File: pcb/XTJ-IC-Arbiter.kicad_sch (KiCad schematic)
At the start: 34 parts, among them J3 DTM13-12PA-R008, SW1 SW_DIP_x01, SW2 SW_DIP_x01, U1 LM2672N-5.0, U3 Teensy4.0, U4 MCP2562-H-P, U5 SP723ABG

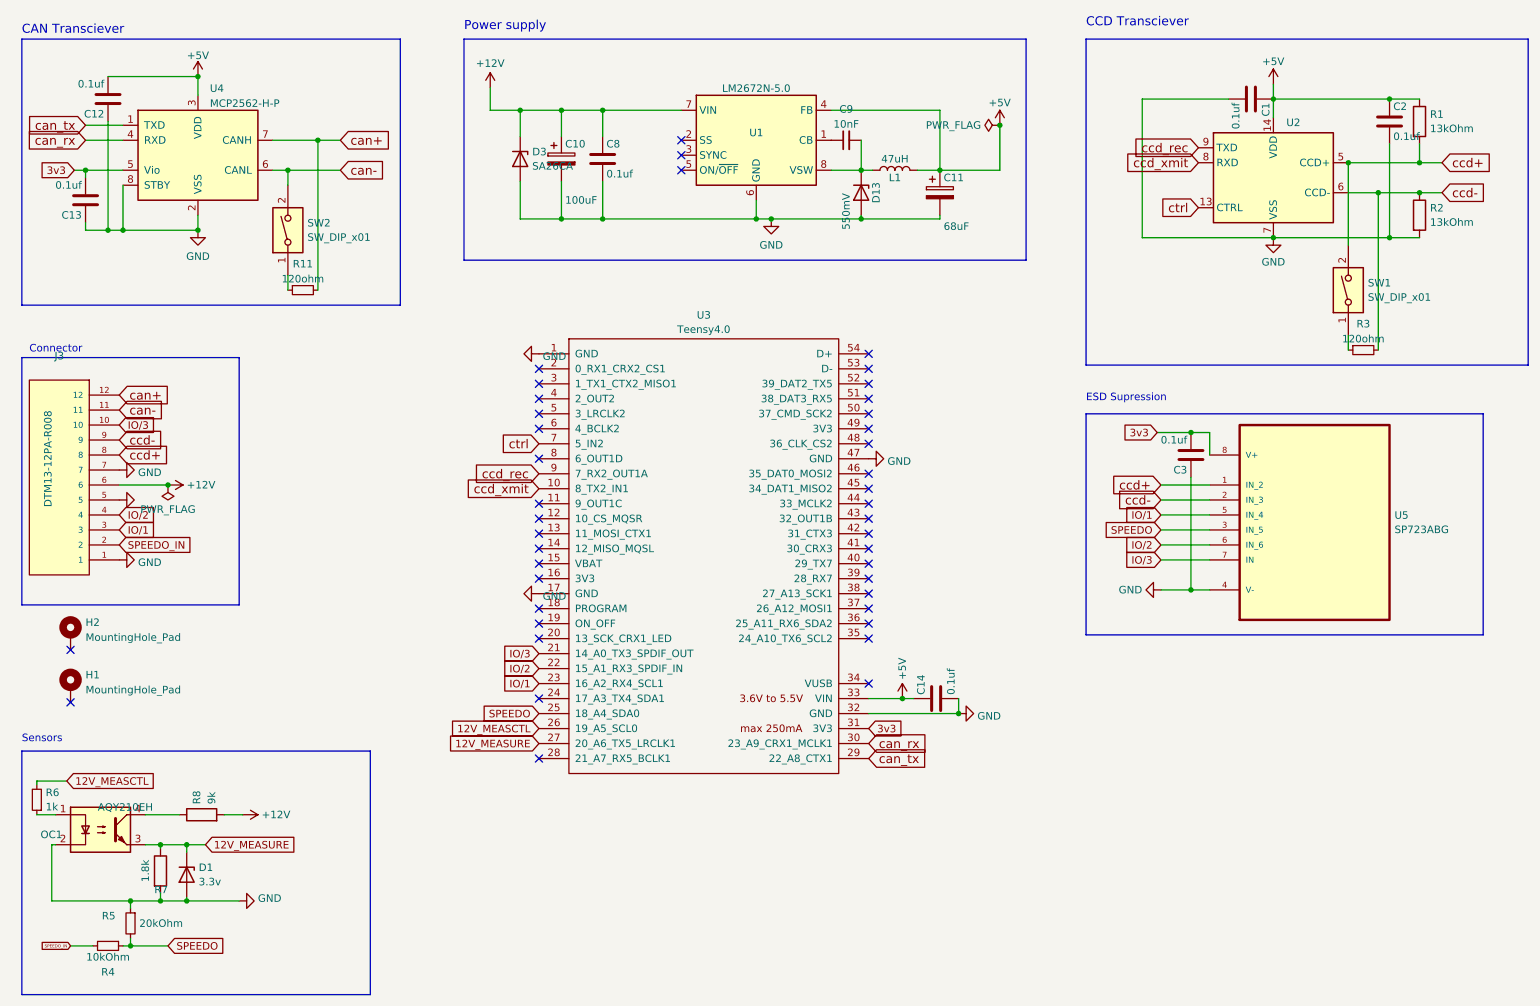
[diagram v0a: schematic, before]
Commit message: ugly but functional
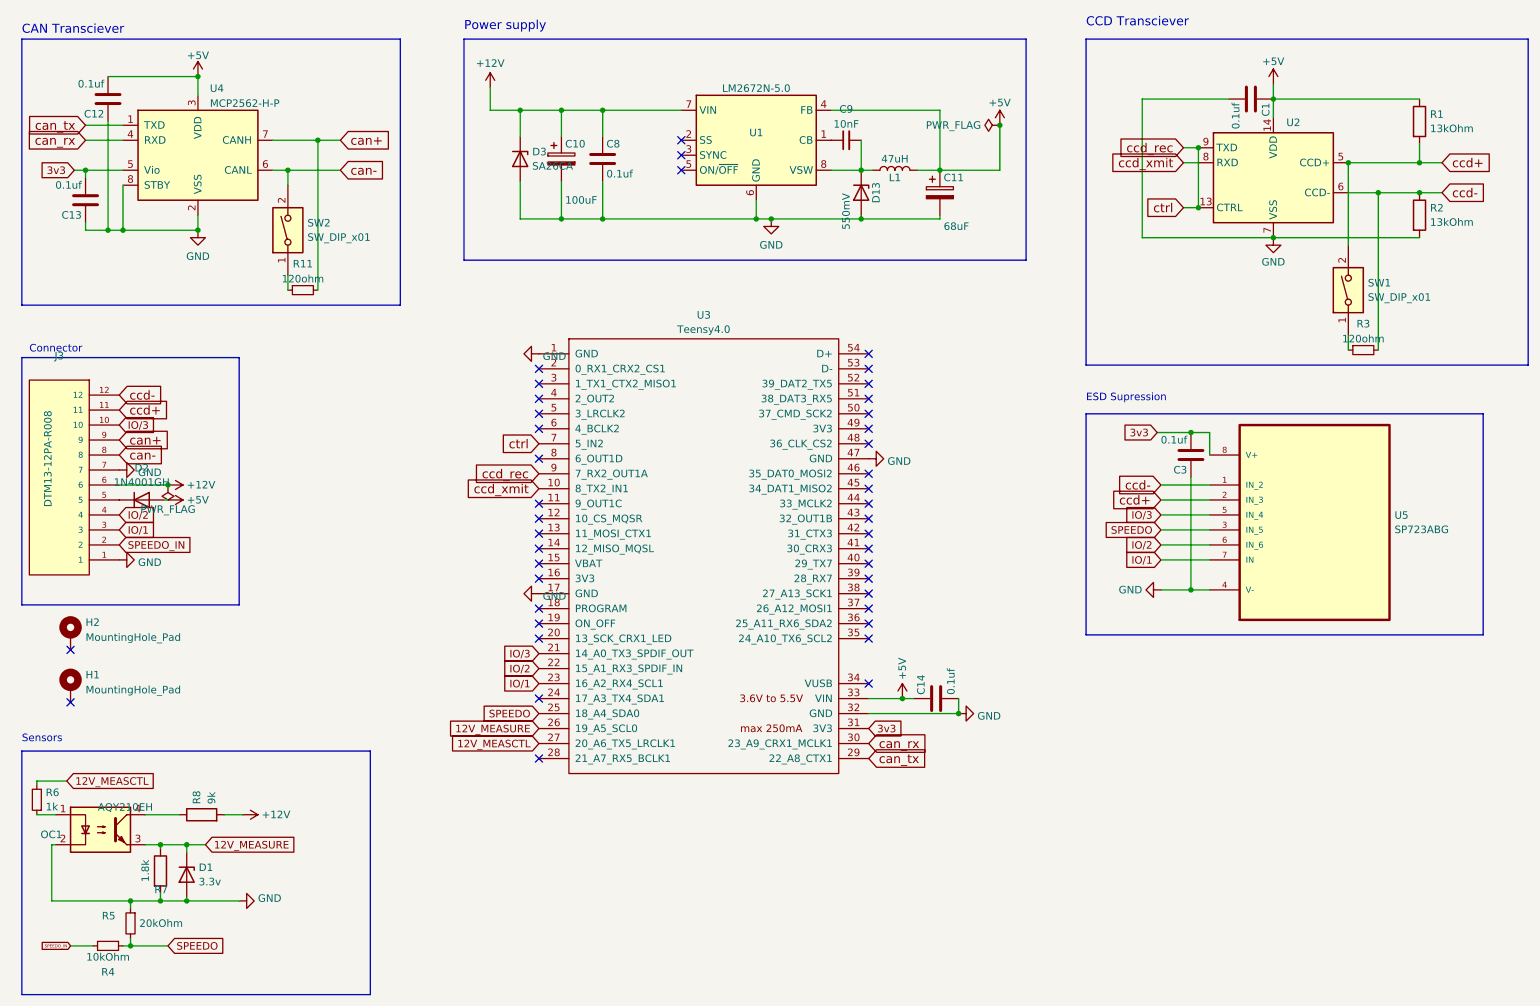
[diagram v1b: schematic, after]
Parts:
- removed C2: 0.1uf, Capacitor_THT:C_Disc_D3.8mm_W2.6mm_P2.50mm, symbol Device:C
- added D2: 1N4001GH, Diode_THT:D_DO-41_SOD81_P7.62mm_Horizontal, symbol Device:D
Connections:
- net ctrl is gone; now on net ccd_rec: U2.13 (CTRL), U3.7 (5_IN2)
- net +5V: now also D2.2 (A)
- net 12V_MEASCTL: now also U3.27 (20_A6_TX5_LRCLK1); no longer U3.26 (19_A5_SCL0)
- net 12V_MEASURE: now also U3.26 (19_A5_SCL0); no longer U3.27 (20_A6_TX5_LRCLK1)
- net GND: no longer J3.5
- net IO/1: now also U5.7 (IN); no longer U5.5 (IN_4)
- net IO/3: now also U5.5 (IN_4); no longer U5.7 (IN)
- net can+: now also J3.9; no longer J3.12
- net can-: now also J3.8; no longer J3.11
- net ccd+: now also J3.11, U5.2 (IN_3); no longer J3.8, U5.1 (IN_2)
- net ccd-: now also J3.12, U5.1 (IN_2); no longer J3.9, U5.2 (IN_3)
- new net: D2.1 (K), J3.5

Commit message: less ugly
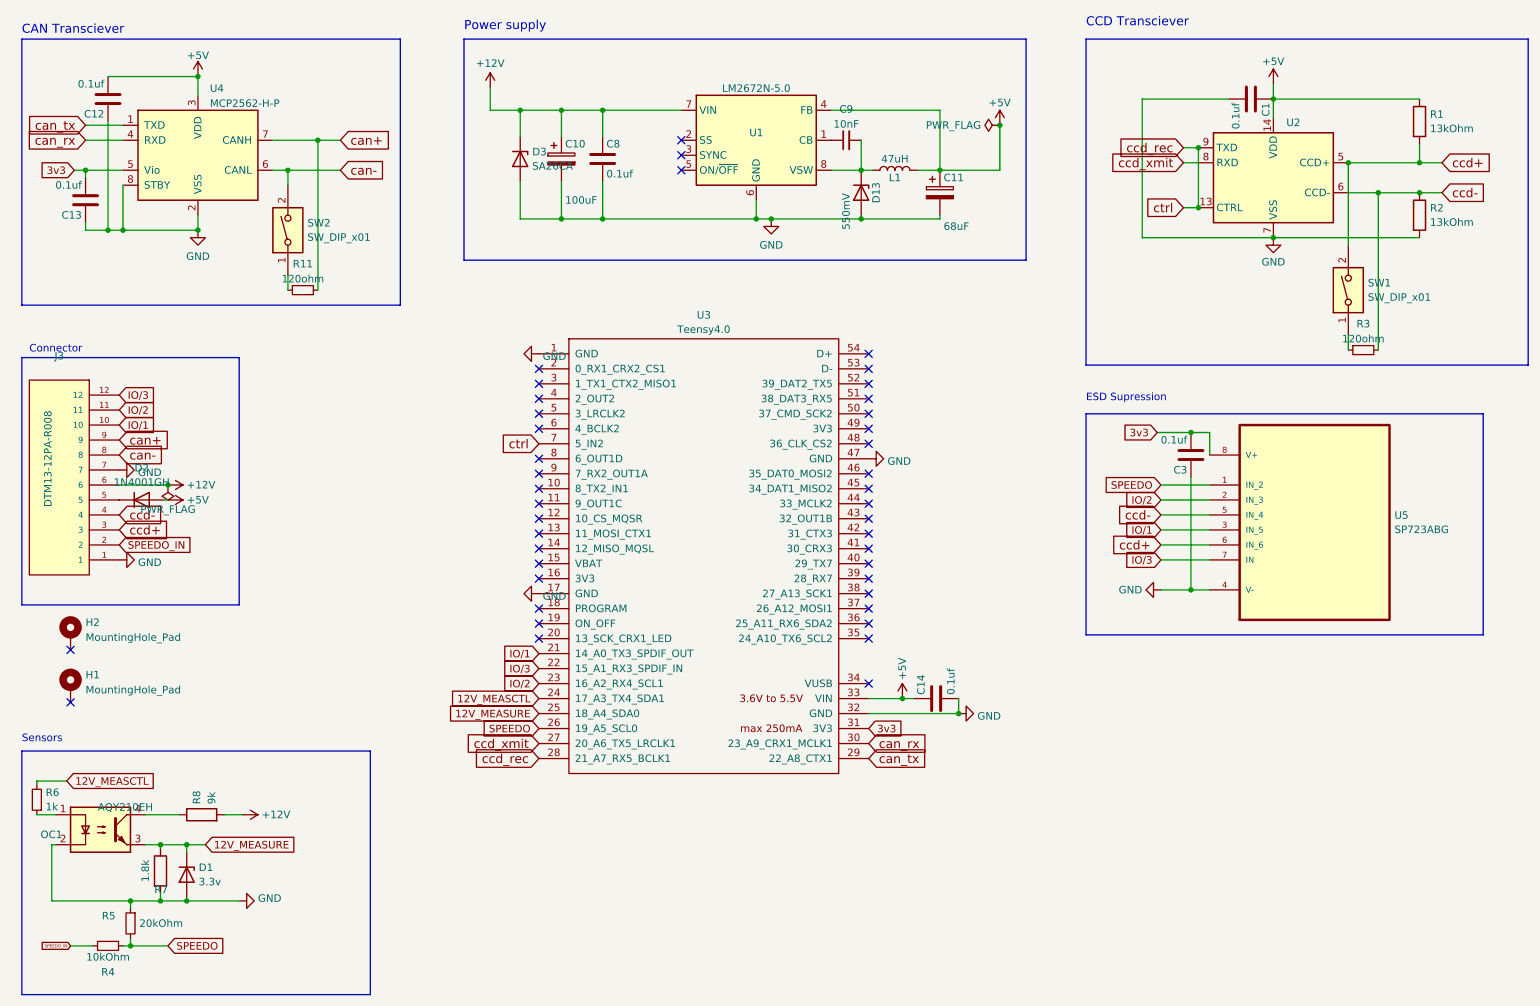
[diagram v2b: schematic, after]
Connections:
- net 12V_MEASCTL: now also U3.24 (17_A3_TX4_SDA1); no longer U3.27 (20_A6_TX5_LRCLK1)
- net 12V_MEASURE: now also U3.25 (18_A4_SDA0); no longer U3.26 (19_A5_SCL0)
- net IO/1: now also J3.10, U3.21 (14_A0_TX3_SPDIF_OUT), U5.3 (IN_5); no longer J3.3, U3.23 (16_A2_RX4_SCL1), U5.7 (IN)
- net IO/2: now also J3.11, U3.23 (16_A2_RX4_SCL1), U5.2 (IN_3); no longer J3.4, U3.22 (15_A1_RX3_SPDIF_IN), U5.6 (IN_6)
- net IO/3: now also J3.12, U3.22 (15_A1_RX3_SPDIF_IN), U5.7 (IN); no longer J3.10, U3.21 (14_A0_TX3_SPDIF_OUT), U5.5 (IN_4)
- net SPEEDO: now also U3.26 (19_A5_SCL0), U5.1 (IN_2); no longer U3.25 (18_A4_SDA0), U5.3 (IN_5)
- net ccd+: now also J3.3, U5.6 (IN_6); no longer J3.11, U5.2 (IN_3)
- net ccd-: now also J3.4, U5.5 (IN_4); no longer J3.12, U5.1 (IN_2)
- net ccd_rec: now also U3.28 (21_A7_RX5_BCLK1); no longer U3.9 (7_RX2_OUT1A)
- net ccd_xmit: now also U3.27 (20_A6_TX5_LRCLK1); no longer U3.10 (8_TX2_IN1)

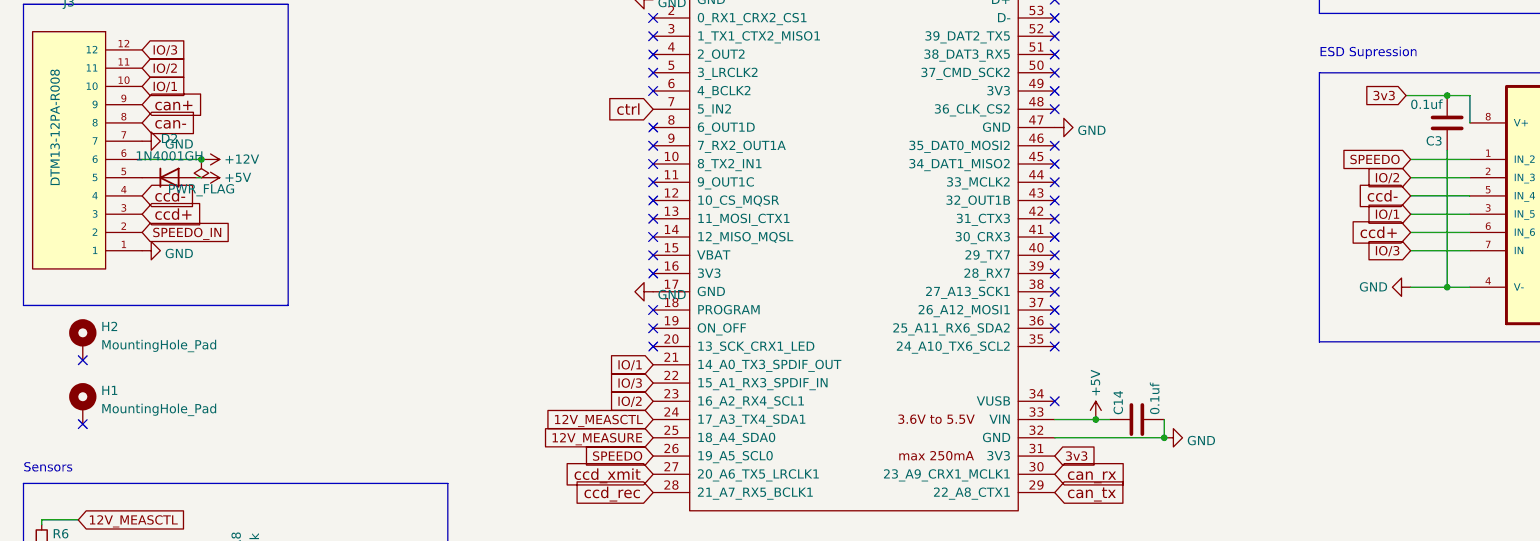
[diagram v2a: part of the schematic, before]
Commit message: polish, text
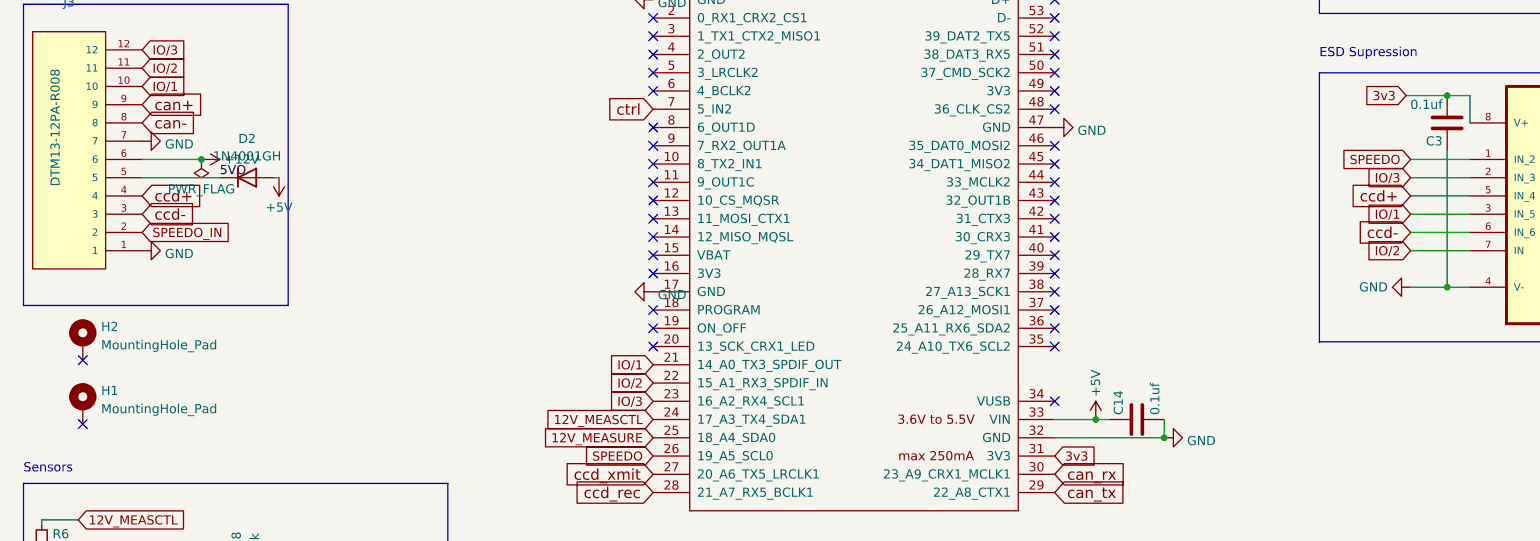
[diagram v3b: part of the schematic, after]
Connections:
- net IO/2: now also U3.22 (15_A1_RX3_SPDIF_IN), U5.7 (IN); no longer U3.23 (16_A2_RX4_SCL1), U5.2 (IN_3)
- net IO/3: now also U3.23 (16_A2_RX4_SCL1), U5.2 (IN_3); no longer U3.22 (15_A1_RX3_SPDIF_IN), U5.7 (IN)
- net ccd+: now also J3.4, U5.5 (IN_4); no longer J3.3, U5.6 (IN_6)
- net ccd-: now also J3.3, U5.6 (IN_6); no longer J3.4, U5.5 (IN_4)
- net 5VO: now reaches D2.1 (K), J3.5
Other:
- moved on the sheet: D2
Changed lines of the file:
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@@
+    (stroke (width 0) (type default))
+  )
+  (wire (pts (xy 45.085 102.235) (xy 34.29 102.235))
     (stroke (width 0) (type default))
   )
@@
     (stroke (width 0) (type default))
   )
-  (wire (pts (xy 41.91 102.235) (xy 42.545 102.235))
+  (wire (pts (xy 52.705 102.235) (xy 53.34 102.235))
     (stroke (width 0) (type default))
   )
@@
   )
   (text "Connector" (at 19.05 77.47 0)
+    (effects (font (size 1.27 1.27)) (justify left bottom))
+  )
+  (label "5VO" (at 45.085 102.235 0) (fields_autoplaced)
     (effects (font (size 1.27 1.27)) (justify left bottom))
   )
@@
     )
   )
-  (global_label "IO{slash}2" (shape input) (at 105.41 133.35 180) (fields_autoplaced)
+  (global_label "IO{slash}2" (shape input) (at 105.41 130.81 180) (fields_autoplaced)
     (effects (font (size 1.27 1.27)) (justify right))
-    (property "Intersheetrefs" "${INTERSHEET_REFS}" (at 98.5217 133.4294 0)
+    (property "Intersheetrefs" "${INTERSHEET_REFS}" (at 98.5217 130.8894 0)
       (effects (font (size 1.27 1.27)) (justify right) hide)
     )
@@
     )
   )
-  (global_label "ccd+" (shape input) (at 210.82 109.855 180) (fields_autoplaced)
+  (global_label "ccd+" (shape input) (at 210.82 104.775 180) (fields_autoplaced)
     (effects (font (size 1.524 1.524)) (justify right))
-    (property "Intersheetrefs" "${INTERSHEET_REFS}" (at 201.3599 109.855 0)
+    (property "Intersheetrefs" "${INTERSHEET_REFS}" (at 201.3599 104.775 0)
       (effects (font (size 1.27 1.27)) (justify right) hide)
     )
@@
     )
   )
-  (global_label "ccd+" (shape input) (at 34.29 107.315 0) (fields_autoplaced)
+  (global_label "ccd+" (shape input) (at 34.29 104.775 0) (fields_autoplaced)
     (effects (font (size 1.524 1.524)) (justify left))
-    (property "Intersheetrefs" "${INTERSHEET_REFS}" (at 256.54 212.725 0)
+    (property "Intersheetrefs" "${INTERSHEET_REFS}" (at 256.54 210.185 0)
       (effects (font (size 1.27 1.27)) hide)
     )
@@
     )
   )
-  (global_label "IO{slash}3" (shape input) (at 105.41 130.81 180) (fields_autoplaced)
+  (global_label "IO{slash}3" (shape input) (at 105.41 133.35 180) (fields_autoplaced)
     (effects (font (size 1.27 1.27)) (justify right))
-    (property "Intersheetrefs" "${INTERSHEET_REFS}" (at 98.5217 130.8894 0)
+    (property "Intersheetrefs" "${INTERSHEET_REFS}" (at 98.5217 133.4294 0)
       (effects (font (size 1.27 1.27)) (justify right) hide)
     )
@@
     )
   )
-  (global_label "IO{slash}3" (shape input) (at 210.82 112.395 180) (fields_autoplaced)
+  (global_label "IO{slash}3" (shape input) (at 210.82 102.235 180) (fields_autoplaced)
     (effects (font (size 1.27 1.27)) (justify right))
-    (property "Intersheetrefs" "${INTERSHEET_REFS}" (at 203.3595 112.395 0)
+    (property "Intersheetrefs" "${INTERSHEET_REFS}" (at 203.3595 102.235 0)
       (effects (font (size 1.27 1.27)) (justify right) hide)
     )
@@
     )
   )
-  (global_label "IO{slash}2" (shape input) (at 210.82 102.235 180) (fields_autoplaced)
+  (global_label "IO{slash}2" (shape input) (at 210.82 112.395 180) (fields_autoplaced)
     (effects (font (size 1.27 1.27)) (justify right))
-    (property "Intersheetrefs" "${INTERSHEET_REFS}" (at 203.3595 102.235 0)
+    (property "Intersheetrefs" "${INTERSHEET_REFS}" (at 203.3595 112.395 0)
       (effects (font (size 1.27 1.27)) (justify right) hide)
     )
@@
     )
   )
-  (global_label "ccd-" (shape input) (at 210.82 104.775 180) (fields_autoplaced)
+  (global_label "ccd-" (shape input) (at 210.82 109.855 180) (fields_autoplaced)
     (effects (font (size 1.524 1.524)) (justify right))
-    (property "Intersheetrefs" "${INTERSHEET_REFS}" (at 201.3599 104.775 0)
+    (property "Intersheetrefs" "${INTERSHEET_REFS}" (at 201.3599 109.855 0)
       (effects (font (size 1.27 1.27)) (justify right) hide)
     )
@@
     )
   )
-  (global_label "ccd-" (shape input) (at 34.29 104.775 0) (fields_autoplaced)
+  (global_label "ccd-" (shape input) (at 34.29 107.315 0) (fields_autoplaced)
     (effects (font (size 1.524 1.524)) (justify left))
-    (property "Intersheetrefs" "${INTERSHEET_REFS}" (at 260.35 241.935 0)
+    (property "Intersheetrefs" "${INTERSHEET_REFS}" (at 260.35 244.475 0)
       (effects (font (size 1.27 1.27)) hide)
     )
@@
     )
   )
-  (symbol (lib_id "power:+5V") (at 42.545 102.235 270) (unit 1)
-    (in_bom yes) (on_board yes) (dnp no) (fields_autoplaced)
-    (property "Reference" "#PWR012" (at 38.735 102.235 0)
-      (effects (font (size 1.27 1.27)) hide)
-    )
-    (property "Value" "+5V" (at 45.72 102.235 90)
-      (effects (font (size 1.27 1.27)) (justify left))
-    )
-    (property "Footprint" "" (at 42.545 102.235 0)
-      (effects (font (size 1.27 1.27)) hide)
-    )
-    (property "Datasheet" "" (at 42.545 102.235 0)
+  (symbol (lib_id "power:+5V") (at 53.34 102.235 180) (unit 1)
+    (in_bom yes) (on_board yes) (dnp no) (fields_autoplaced)
+    (property "Reference" "#PWR012" (at 53.34 98.425 0)
+      (effects (font (size 1.27 1.27)) hide)
+    )
+    (property "Value" "+5V" (at 53.34 106.3681 0)
+      (effects (font (size 1.27 1.27)))
+    )
+    (property "Footprint" "" (at 53.34 102.235 0)
+      (effects (font (size 1.27 1.27)) hide)
+    )
+    (property "Datasheet" "" (at 53.34 102.235 0)
       (effects (font (size 1.27 1.27)) hide)
     )
@@
     )
   )
-  (symbol (lib_id "Device:D") (at 38.1 102.235 0) (unit 1)
-    (in_bom yes) (on_board yes) (dnp no) (fields_autoplaced)
-    (property "Reference" "D2" (at 38.1 96.8207 0)
-      (effects (font (size 1.27 1.27)))
-    )
-    (property "Value" "1N4001GH " (at 38.1 99.2449 0)
-      (effects (font (size 1.27 1.27)))
-    )
-    (property "Footprint" "Diode_THT:D_DO-41_SOD81_P7.62mm_Horizontal" (at 38.1 102.235 0)
-      (effects (font (size 1.27 1.27)) hide)
-    )
-    (property "Datasheet" "~" (at 38.1 102.235 0)
-      (effects (font (size 1.27 1.27)) hide)
-    )
-    (property "Sim.Device" "D" (at 38.1 102.235 0)
-      (effects (font (size 1.27 1.27)) hide)
-    )
-    (property "Sim.Pins" "1=K 2=A" (at 38.1 102.235 0)
-      (effects (font (size 1.27 1.27)) hide)
-    )
+  (symbol (lib_id "Device:D") (at 48.895 102.235 0) (unit 1)
+    (in_bom yes) (on_board yes) (dnp no) (fields_autoplaced)
+    (property "Reference" "D2" (at 48.895 96.8207 0)
+      (effects (font (size 1.27 1.27)))
+    )
+    (property "Value" "1N4001GH " (at 48.895 99.2449 0)
+      (effects (font (size 1.27 1.27)))
+    )
+    (property "Footprint" "Diode_THT:D_DO-41_SOD81_P7.62mm_Horizontal" (at 48.895 102.235 0)
+      (effects (font (size 1.27 1.27)) hide)
+    )
+    (property "Datasheet" "~" (at 48.895 102.235 0)
+      (effects (font (size 1.27 1.27)) hide)
+    )
+    (property "Sim.Device" "D" (at 48.895 102.235 0)
+      (effects (font (size 1.27 1.27)) hide)
+    )
+    (property "Sim.Pins" "1=K 2=A" (at 48.895 102.235 0)
+      (effects (font (size 1.27 1.27)) hide)
+    )
